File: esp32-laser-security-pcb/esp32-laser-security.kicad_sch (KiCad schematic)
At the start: 5 parts, among them J1 Conn_01x06, SW1 SW_Push

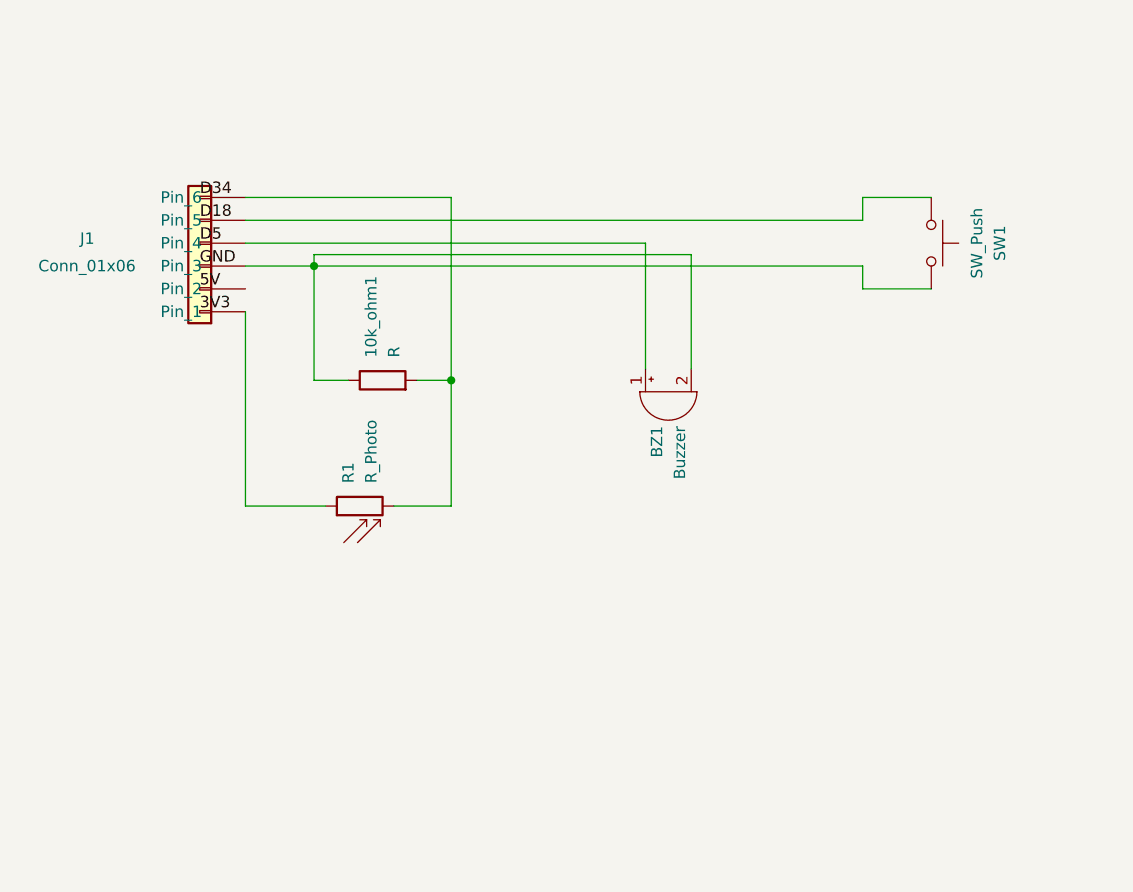
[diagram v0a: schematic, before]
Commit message: added mount & updated pcb
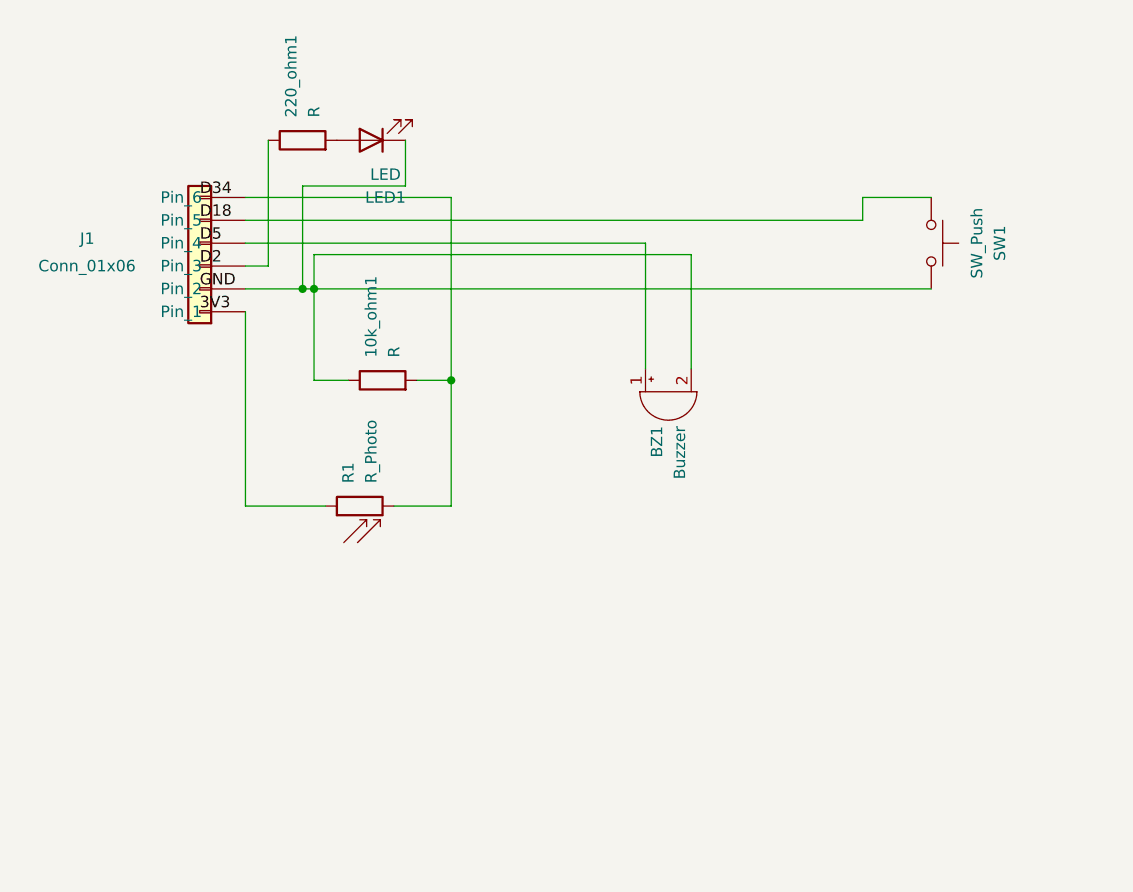
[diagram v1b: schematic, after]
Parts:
- added 220_ohm1: R, Resistor_THT:R_Axial_DIN0207_L6.3mm_D2.5mm_P7.62mm_Horizontal, symbol Device:R
- added LED1: LED, LED_THT:LED_D5.0mm, symbol Device:LED
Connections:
- net at 10k_ohm1.1, BZ1.2 (-), SW1.2: now also J1.2 (Pin_2), LED1.1 (K); no longer J1.3 (Pin_3)
- new net: 220_ohm1.1, J1.3 (Pin_3)
- new net: 220_ohm1.2, LED1.2 (A)
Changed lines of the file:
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@@
 	(paper "A4")
 	(junction
-		(at 134.62 66.04)
+		(at 134.62 68.58)
 		(diameter 0)
 		(color 0 0 0 0)
@@
 		(color 0 0 0 0)
 	)
+	(junction
+		(at 133.35 68.58)
+		(diameter 0)
+		(color 0 0 0 0)
+	)
+	(wire
+		(pts
+			(xy 133.35 68.58) (xy 134.62 68.58)
+		)
+		(stroke
+			(width 0)
+			(type default)
+		)
+	)
 	(wire
 		(pts
@@
 	(wire
 		(pts
-			(xy 134.62 66.04) (xy 134.62 78.74)
+			(xy 129.54 52.07) (xy 129.54 66.04)
+		)
+		(stroke
+			(width 0)
+			(type default)
+		)
+	)
+	(wire
+		(pts
+			(xy 134.62 68.58) (xy 134.62 78.74)
 		)
 		(stroke
@@
 	(wire
 		(pts
-			(xy 127 66.04) (xy 134.62 66.04)
-		)
-		(stroke
-			(width 0)
-			(type default)
-		)
-	)
-	(wire
-		(pts
 			(xy 127 60.96) (xy 195.58 60.96)
 		)
@@
 	(wire
 		(pts
+			(xy 129.54 66.04) (xy 127 66.04)
+		)
+		(stroke
+			(width 0)
+			(type default)
+		)
+	)
+	(wire
+		(pts
 			(xy 127 92.71) (xy 127 71.12)
 		)
@@
 	(wire
 		(pts
-			(xy 134.62 64.77) (xy 134.62 66.04)
+			(xy 134.62 64.77) (xy 134.62 68.58)
 		)
 		(stroke
@@
 	(wire
 		(pts
+			(xy 127 68.58) (xy 133.35 68.58)
+		)
+		(stroke
+			(width 0)
+			(type default)
+		)
+	)
+	(wire
+		(pts
 			(xy 149.86 78.74) (xy 149.86 92.71)
 		)
@@
 	(wire
 		(pts
+			(xy 133.35 57.15) (xy 133.35 68.58)
+		)
+		(stroke
+			(width 0)
+			(type default)
+		)
+	)
+	(wire
+		(pts
 			(xy 134.62 78.74) (xy 138.43 78.74)
 		)
@@
 	(wire
 		(pts
-			(xy 134.62 66.04) (xy 195.58 66.04)
+			(xy 144.78 52.07) (xy 144.78 57.15)
+		)
+		(stroke
+			(width 0)
+			(type default)
+		)
+	)
+	(wire
+		(pts
+			(xy 134.62 68.58) (xy 203.2 68.58)
 		)
 		(stroke
@@
 	(wire
 		(pts
-			(xy 195.58 66.04) (xy 195.58 68.58)
-		)
-		(stroke
-			(width 0)
-			(type default)
-		)
-	)
-	(wire
-		(pts
-			(xy 195.58 68.58) (xy 203.2 68.58)
+			(xy 144.78 57.15) (xy 133.35 57.15)
 		)
 		(stroke
@@
 		)
 	)
-	(label "5V"
+	(label "GND"
 		(at 121.92 68.58 0)
 		(effects
@@
 		)
 	)
-	(label "GND"
+	(label "D2"
 		(at 121.92 66.04 0)
 		(effects
@@
 	)
 	(symbol
+		(lib_id "Device:R")
+		(at 133.35 52.07 90)
+		(unit 1)
+		(body_style 1)
+		(exclude_from_sim no)
+		(in_bom yes)
+		(on_board yes)
+		(in_pos_files yes)
+		(dnp no)
+		(fields_autoplaced yes)
+		(property "Reference" "220_ohm1"
+			(at 132.0799 49.53 0)
+			(show_name no)
+			(do_not_autoplace no)
+			(effects
+				(font
+					(size 1.27 1.27)
+				)
+				(justify left)
+			)
+		)
+		(property "Value" "R"
+			(at 134.6199 49.53 0)
+			(show_name no)
+			(do_not_autoplace no)
+			(effects
+				(font
+					(size 1.27 1.27)
+				)
+				(justify left)
+			)
+		)
+		(property "Footprint" "Resistor_THT:R_Axial_DIN0207_L6.3mm_D2.5mm_P7.62mm_Horizontal"
+			(at 133.35 53.848 90)
+			(hide yes)
+			(show_name no)
+			(do_not_autoplace no)
+			(effects
+				(font
+					(size 1.27 1.27)
+				)
+			)
+		)
+		(property "Datasheet" ""
+			(at 133.35 52.07 0)
+			(hide yes)
+			(show_name no)
+			(do_not_autoplace no)
+			(effects
+				(font
+					(size 1.27 1.27)
+				)
+			)
+		)
+		(property "Description" "Resistor"
+			(at 133.35 52.07 0)
+			(hide yes)
+			(show_name no)
+			(do_not_autoplace no)
+			(effects
+				(font
+					(size 1.27 1.27)
+				)
+			)
+		)
+		(pin "1"
+		)
+		(pin "2"
+		)
+		(instances
+			(project "esp32-laser-security"
+				(path "/46dd9cca-a9f6-46c6-90d0-bd2585ef2119"
+					(reference "220_ohm1")
+					(unit 1)
+				)
+			)
+		)
+	)
+	(symbol
 		(lib_id "Connector_Generic:Conn_01x06")
 		(at 121.92 66.04 180)
@@
 					(unit 1)
 				)
+			)
+		)
+	)
+	(symbol
+		(lib_id "Device:LED")
+		(at 140.97 52.07 180)
+		(unit 1)
+		(body_style 1)
+		(exclude_from_sim no)
+		(in_bom yes)
+		(on_board yes)
+		(in_pos_files yes)
+		(dnp no)
+		(fields_autoplaced yes)
+		(property "Reference" "LED1"
+			(at 142.5575 58.42 0)
+			(show_name no)
+			(do_not_autoplace no)
+			(effects
+				(font
+					(size 1.27 1.27)
+				)
+			)
+		)
+		(property "Value" "LED"
+			(at 142.5575 55.88 0)
+			(show_name no)
+			(do_not_autoplace no)
+			(effects
+				(font
+					(size 1.27 1.27)
+				)
+			)
+		)
+		(property "Footprint" "LED_THT:LED_D5.0mm"
+			(at 140.97 52.07 0)
+			(hide yes)
+			(show_name no)
+			(do_not_autoplace no)
+			(effects
+				(font
+					(size 1.27 1.27)
+				)
+			)
+		)
+		(property "Datasheet" ""
+			(at 140.97 52.07 0)
+			(hide yes)
+			(show_name no)
+			(do_not_autoplace no)
+			(effects
+				(font
+					(size 1.27 1.27)
+				)
+			)
+		)
+		(property "Description" "Light emitting diode"
+			(at 140.97 52.07 0)
+			(hide yes)
+			(show_name no)
+			(do_not_autoplace no)
+			(effects
+				(font
+					(size 1.27 1.27)
+				)
+			)
+		)
+		(property "Sim.Pins" "1=K 2=A"
+			(at 140.97 52.07 0)
+			(hide yes)
+			(show_name no)
+			(do_not_autoplace no)
+			(effects
+				(font
+					(size 1.27 1.27)
+				)
+			)
+		)
+		(pin "2"
+		)
+		(pin "1"
+		)
+		(instances
+			(project "esp32-laser-security"
+				(path "/46dd9cca-a9f6-46c6-90d0-bd2585ef2119"
+					(reference "LED1")
+					(unit 1)
+				)

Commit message: updated pcb
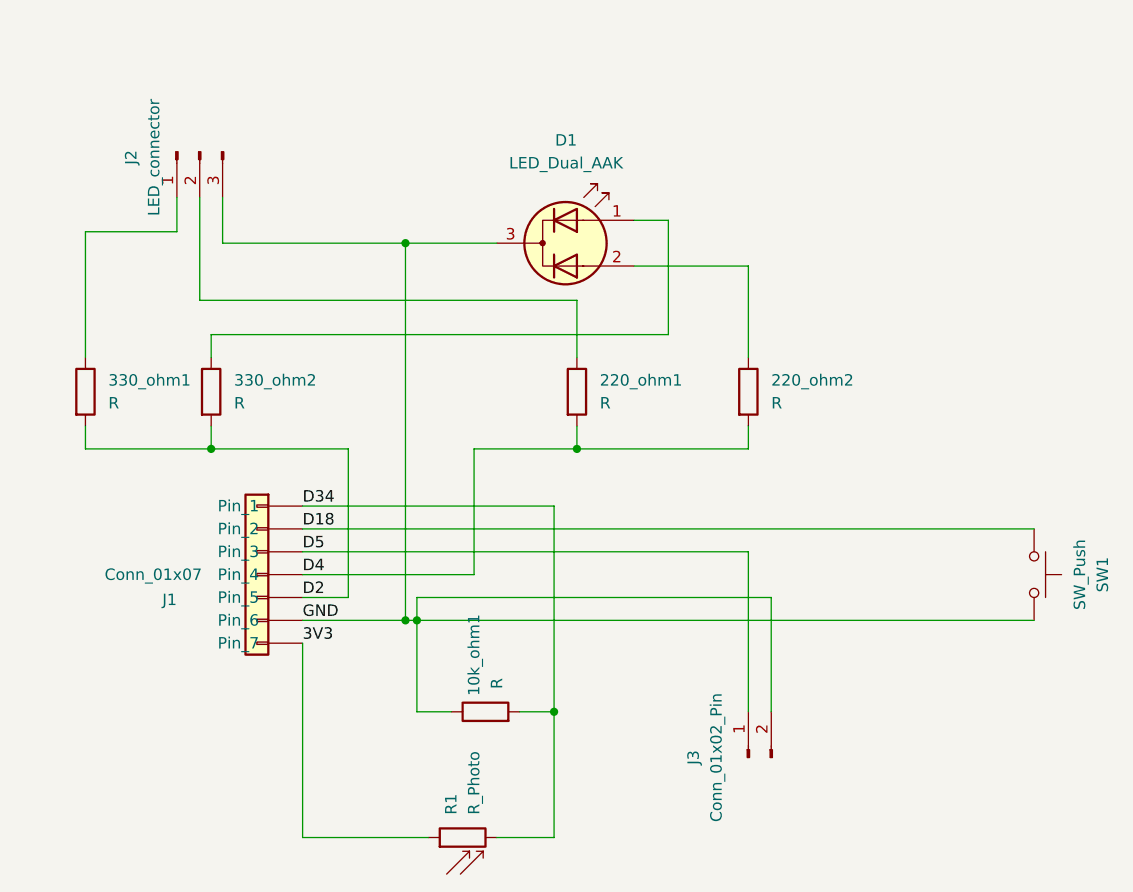
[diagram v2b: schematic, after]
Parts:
- removed BZ1: Buzzer, Buzzer_Beeper:Buzzer_12x9.5RM7.6, symbol Device:Buzzer
- removed J1: Conn_01x06, Connector_PinHeader_2.54mm:PinHeader_1x06_P2.54mm_Vertical, symbol Connector_Generic:Conn_01x06
- removed LED1: LED, LED_THT:LED_D5.0mm, symbol Device:LED
- added 220_ohm2, 330_ohm1, 330_ohm2: R, Resistor_THT:R_Axial_DIN0207_L6.3mm_D2.5mm_P7.62mm_Horizontal, symbol Device:R
- added D1: LED_Dual_AAK, LED_THT:LED_D5.0mm-3, symbol Device:LED_Dual_AAK
- added J1: Conn_01x07, Connector_PinHeader_2.54mm:PinHeader_1x07_P2.54mm_Vertical, symbol Connector_Generic:Conn_01x07
- added J2: LED_connector, Connector_JST:JST_XH_B3B-XH-AM_1x03_P2.50mm_Vertical, symbol Connector:Conn_01x03_Pin
- added J3: Conn_01x02_Pin, TerminalBlock:TerminalBlock_MaiXu_MX126-5.0-02P_1x02_P5.00mm, symbol Connector:Conn_01x02_Pin
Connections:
- net 3V3: now also R1.1, J1.7 (Pin_7)
- net D18: now also SW1.1, J1.2 (Pin_2)
- net D2: now also 330_ohm1.2, 330_ohm2.2, J1.5 (Pin_5)
- net D34: now also 10k_ohm1.2, R1.2, J1.1 (Pin_1)
- net D5: now also J1.3 (Pin_3), J3.1 (Pin_1)
- net GND: now also 10k_ohm1.1, SW1.2, D1.3 (K), J1.6 (Pin_6), J2.3 (Pin_3), J3.2 (Pin_2)
- net at 220_ohm1.1: now also J2.2 (Pin_2)
- net D4: now reaches 220_ohm1.2
- net D4: now also 220_ohm2.2, J1.4 (Pin_4)
- new net: 330_ohm1.1, J2.1 (Pin_1)
- new net: 220_ohm2.1, D1.2 (A2)
- new net: 330_ohm2.1, D1.1 (A1)
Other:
- moved on the sheet: 10k_ohm1, R1, SW1
